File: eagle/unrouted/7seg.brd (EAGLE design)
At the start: 43.2 x 33 mm, 14 parts, among them J1 CONN-8P, J2 CONN-4P-4P

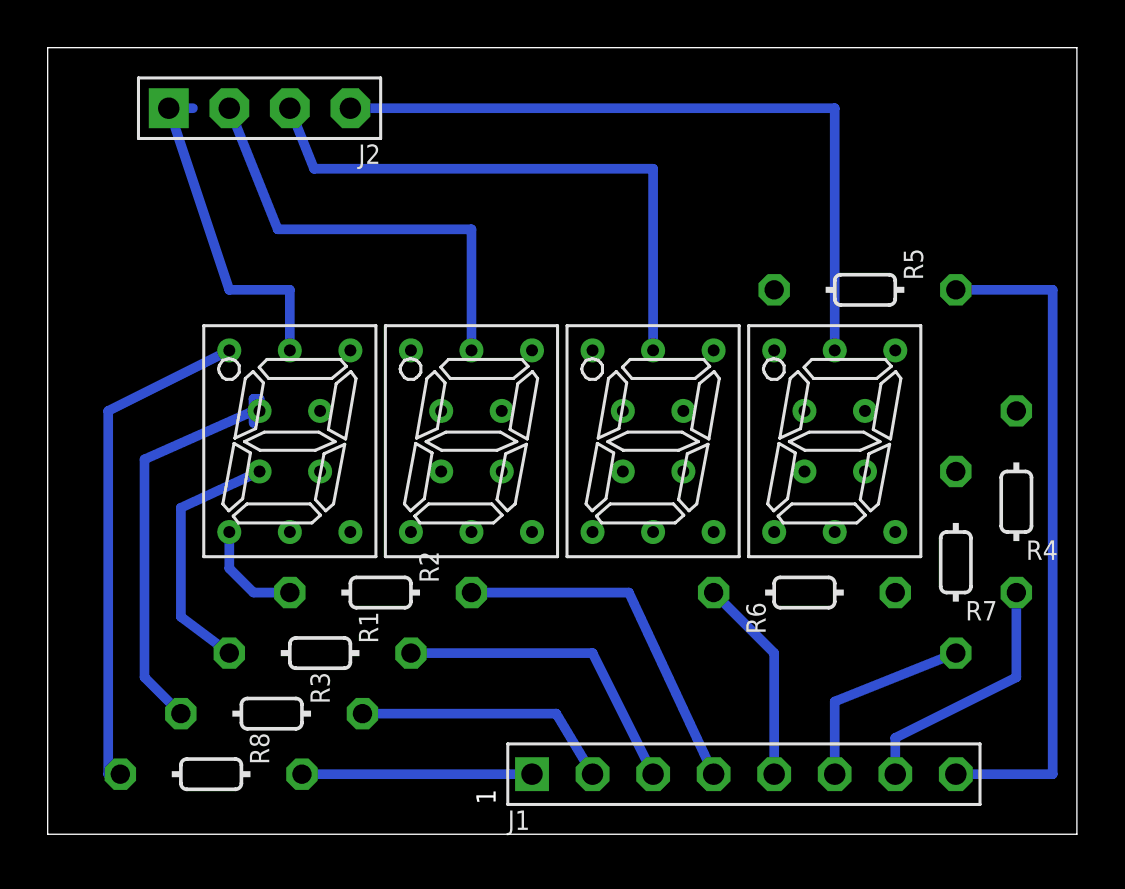
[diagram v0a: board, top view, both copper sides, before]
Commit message: ...
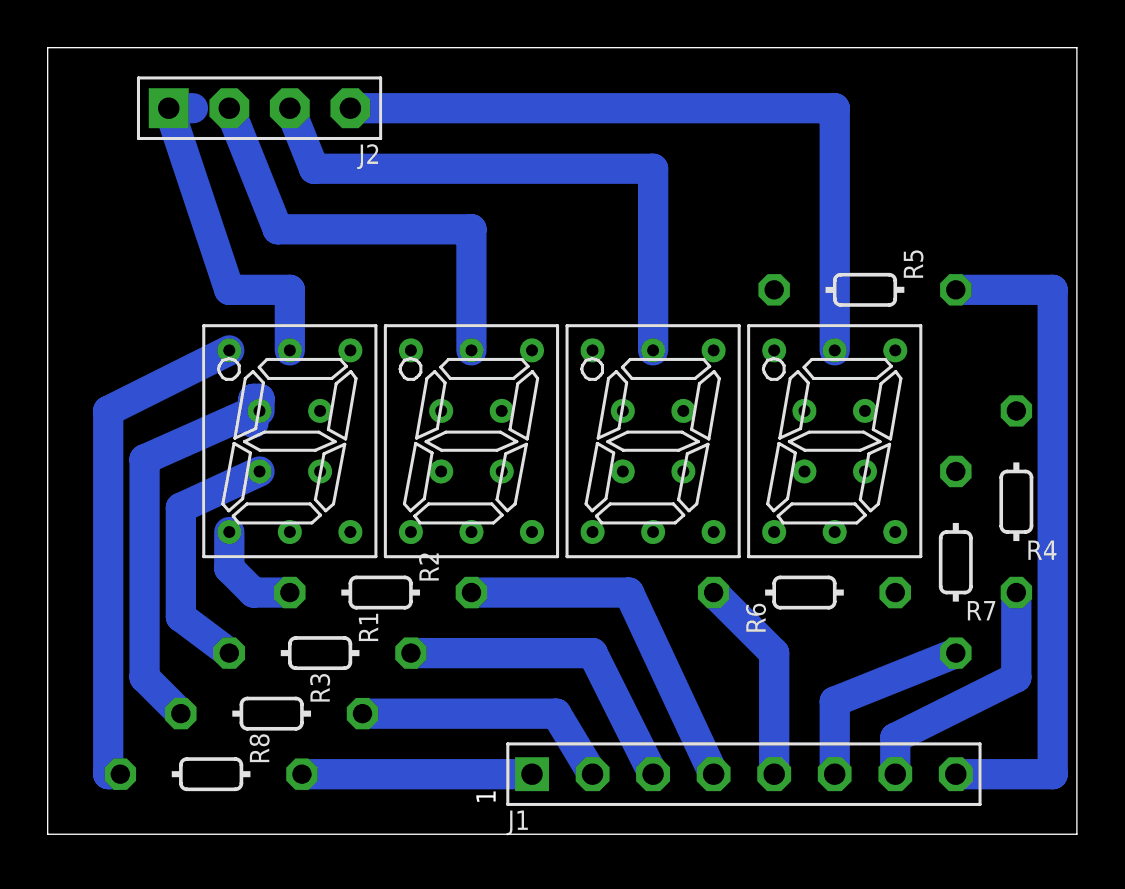
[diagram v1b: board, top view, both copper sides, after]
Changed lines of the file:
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@@
 <contactref element="U$1" pad="8"/>
 <contactref element="J2" pad="1"/>
-<wire x1="6.096" y1="30.48" x2="5.08" y2="30.48" width="0.4064" layer="16"/>
-<wire x1="5.08" y1="30.48" x2="7.62" y2="22.86" width="0.4064" layer="16"/>
-<wire x1="7.62" y1="22.86" x2="10.16" y2="22.86" width="0.4064" layer="16"/>
-<wire x1="10.16" y1="22.86" x2="10.16" y2="20.32" width="0.4064" layer="16"/>
+<wire x1="6.096" y1="30.48" x2="5.08" y2="30.48" width="1.27" layer="16"/>
+<wire x1="5.08" y1="30.48" x2="7.62" y2="22.86" width="1.27" layer="16"/>
+<wire x1="7.62" y1="22.86" x2="10.16" y2="22.86" width="1.27" layer="16"/>
+<wire x1="10.16" y1="22.86" x2="10.16" y2="20.32" width="1.27" layer="16"/>
 <wire x1="10.16" y1="12.7" x2="10.16" y2="20.32" width="0" layer="19" extent="1-1"/>
 </signal>
@@
 <contactref element="U$2" pad="8"/>
 <contactref element="J2" pad="2"/>
-<wire x1="7.62" y1="30.48" x2="9.652" y2="25.4" width="0.4064" layer="16"/>
-<wire x1="9.652" y1="25.4" x2="17.78" y2="25.4" width="0.4064" layer="16"/>
-<wire x1="17.78" y1="25.4" x2="17.78" y2="20.32" width="0.4064" layer="16"/>
+<wire x1="7.62" y1="30.48" x2="9.652" y2="25.4" width="1.27" layer="16"/>
+<wire x1="9.652" y1="25.4" x2="17.78" y2="25.4" width="1.27" layer="16"/>
+<wire x1="17.78" y1="25.4" x2="17.78" y2="20.32" width="1.27" layer="16"/>
 <wire x1="17.78" y1="12.7" x2="17.78" y2="20.32" width="0" layer="19" extent="1-1"/>
 </signal>
@@
 <contactref element="U$3" pad="8"/>
 <contactref element="J2" pad="3"/>
-<wire x1="10.16" y1="30.48" x2="11.176" y2="27.94" width="0.4064" layer="16"/>
-<wire x1="11.176" y1="27.94" x2="25.4" y2="27.94" width="0.4064" layer="16"/>
-<wire x1="25.4" y1="27.94" x2="25.4" y2="20.32" width="0.4064" layer="16"/>
+<wire x1="10.16" y1="30.48" x2="11.176" y2="27.94" width="1.27" layer="16"/>
+<wire x1="11.176" y1="27.94" x2="25.4" y2="27.94" width="1.27" layer="16"/>
+<wire x1="25.4" y1="27.94" x2="25.4" y2="20.32" width="1.27" layer="16"/>
 <wire x1="25.4" y1="20.32" x2="25.4" y2="12.7" width="0" layer="19" extent="1-1"/>
 </signal>
@@
 <contactref element="U$4" pad="8"/>
 <contactref element="J2" pad="4"/>
-<wire x1="12.7" y1="30.48" x2="33.02" y2="30.48" width="0.4064" layer="16"/>
-<wire x1="33.02" y1="30.48" x2="33.02" y2="20.32" width="0.4064" layer="16"/>
+<wire x1="12.7" y1="30.48" x2="33.02" y2="30.48" width="1.27" layer="16"/>
+<wire x1="33.02" y1="30.48" x2="33.02" y2="20.32" width="1.27" layer="16"/>
 <wire x1="33.02" y1="20.32" x2="33.02" y2="12.7" width="0" layer="19" extent="1-1"/>
 </signal>
@@
 <contactref element="U$1" pad="5"/>
 <contactref element="R8" pad="2"/>
-<wire x1="3.048" y1="2.54" x2="2.54" y2="2.54" width="0.4064" layer="16"/>
-<wire x1="2.54" y1="2.54" x2="2.54" y2="17.78" width="0.4064" layer="16"/>
-<wire x1="2.54" y1="17.78" x2="7.62" y2="20.32" width="0.4064" layer="16"/>
+<wire x1="3.048" y1="2.54" x2="2.54" y2="2.54" width="1.27" layer="16"/>
+<wire x1="2.54" y1="2.54" x2="2.54" y2="17.78" width="1.27" layer="16"/>
+<wire x1="2.54" y1="17.78" x2="7.62" y2="20.32" width="1.27" layer="16"/>
 <wire x1="22.86" y1="20.32" x2="30.48" y2="20.32" width="0" layer="19" extent="1-1"/>
 <wire x1="15.24" y1="20.32" x2="22.86" y2="20.32" width="0" layer="19" extent="1-1"/>
@@
 <contactref element="U$2" pad="7"/>
 <contactref element="R1" pad="2"/>
-<wire x1="8.89" y1="15.24" x2="5.588" y2="13.716" width="0.4064" layer="16"/>
-<wire x1="5.588" y1="13.716" x2="5.588" y2="9.144" width="0.4064" layer="16"/>
-<wire x1="5.588" y1="9.144" x2="7.62" y2="7.62" width="0.4064" layer="16"/>
+<wire x1="8.89" y1="15.24" x2="5.588" y2="13.716" width="1.27" layer="16"/>
+<wire x1="5.588" y1="13.716" x2="5.588" y2="9.144" width="1.27" layer="16"/>
+<wire x1="5.588" y1="9.144" x2="7.62" y2="7.62" width="1.27" layer="16"/>
 <wire x1="24.13" y1="15.24" x2="31.75" y2="15.24" width="0" layer="19" extent="1-1"/>
 <wire x1="16.51" y1="15.24" x2="24.13" y2="15.24" width="0" layer="19" extent="1-1"/>
@@
 <contactref element="U$2" pad="6"/>
 <contactref element="R2" pad="2"/>
-<wire x1="10.16" y1="10.16" x2="8.636" y2="10.16" width="0.4064" layer="16"/>
-<wire x1="8.636" y1="10.16" x2="7.62" y2="11.176" width="0.4064" layer="16"/>
-<wire x1="7.62" y1="11.176" x2="7.62" y2="12.7" width="0.4064" layer="16"/>
+<wire x1="10.16" y1="10.16" x2="8.636" y2="10.16" width="1.27" layer="16"/>
+<wire x1="8.636" y1="10.16" x2="7.62" y2="11.176" width="1.27" layer="16"/>
+<wire x1="7.62" y1="11.176" x2="7.62" y2="12.7" width="1.27" layer="16"/>
 <wire x1="22.86" y1="12.7" x2="30.48" y2="12.7" width="0" layer="19" extent="1-1"/>
 <wire x1="15.24" y1="12.7" x2="22.86" y2="12.7" width="0" layer="19" extent="1-1"/>
@@
 <contactref element="U$2" pad="4"/>
 <contactref element="R3" pad="2"/>
-<wire x1="5.588" y1="5.08" x2="4.064" y2="6.604" width="0.4064" layer="16"/>
-<wire x1="4.064" y1="6.604" x2="4.064" y2="15.748" width="0.4064" layer="16"/>
-<wire x1="4.064" y1="15.748" x2="8.636" y2="17.78" width="0.4064" layer="16"/>
-<wire x1="8.636" y1="17.78" x2="8.636" y2="17.272" width="0.4064" layer="16"/>
-<wire x1="8.636" y1="17.78" x2="8.636" y2="18.288" width="0.4064" layer="16"/>
-<wire x1="8.636" y1="18.288" x2="8.89" y2="18.288" width="0.4064" layer="16"/>
-<wire x1="8.89" y1="18.288" x2="8.89" y2="17.78" width="0.4064" layer="16"/>
+<wire x1="5.588" y1="5.08" x2="4.064" y2="6.604" width="1.27" layer="16"/>
+<wire x1="4.064" y1="6.604" x2="4.064" y2="15.748" width="1.27" layer="16"/>
+<wire x1="4.064" y1="15.748" x2="8.636" y2="17.78" width="1.27" layer="16"/>
+<wire x1="8.636" y1="17.78" x2="8.636" y2="17.272" width="1.27" layer="16"/>
+<wire x1="8.636" y1="17.78" x2="8.636" y2="18.288" width="1.27" layer="16"/>
+<wire x1="8.636" y1="18.288" x2="8.89" y2="18.288" width="1.27" layer="16"/>
+<wire x1="8.89" y1="18.288" x2="8.89" y2="17.78" width="1.27" layer="16"/>
 <wire x1="24.13" y1="17.78" x2="31.75" y2="17.78" width="0" layer="19" extent="1-1"/>
 <wire x1="16.51" y1="17.78" x2="24.13" y2="17.78" width="0" layer="19" extent="1-1"/>
@@
 <contactref element="R1" pad="1"/>
 <contactref element="J1" pad="3"/>
-<wire x1="15.24" y1="7.62" x2="22.86" y2="7.62" width="0.4064" layer="16"/>
-<wire x1="22.86" y1="7.62" x2="25.4" y2="2.54" width="0.4064" layer="16"/>
+<wire x1="15.24" y1="7.62" x2="22.86" y2="7.62" width="1.27" layer="16"/>
+<wire x1="22.86" y1="7.62" x2="25.4" y2="2.54" width="1.27" layer="16"/>
 </signal>
 <signal name="N$2">
 <contactref element="R2" pad="1"/>
 <contactref element="J1" pad="4"/>
-<wire x1="17.78" y1="10.16" x2="24.384" y2="10.16" width="0.4064" layer="16"/>
-<wire x1="24.384" y1="10.16" x2="27.94" y2="2.54" width="0.4064" layer="16"/>
+<wire x1="17.78" y1="10.16" x2="24.384" y2="10.16" width="1.27" layer="16"/>
+<wire x1="24.384" y1="10.16" x2="27.94" y2="2.54" width="1.27" layer="16"/>
 </signal>
 <signal name="N$3">
 <contactref element="R3" pad="1"/>
 <contactref element="J1" pad="2"/>
-<wire x1="13.208" y1="5.08" x2="21.336" y2="5.08" width="0.4064" layer="16"/>
-<wire x1="21.336" y1="5.08" x2="22.86" y2="2.54" width="0.4064" layer="16"/>
+<wire x1="13.208" y1="5.08" x2="21.336" y2="5.08" width="1.27" layer="16"/>
+<wire x1="21.336" y1="5.08" x2="22.86" y2="2.54" width="1.27" layer="16"/>
 </signal>
 <signal name="N$4">
 <contactref element="R4" pad="1"/>
 <contactref element="J1" pad="7"/>
-<wire x1="35.56" y1="2.54" x2="35.56" y2="4.064" width="0.4064" layer="16"/>
-<wire x1="35.56" y1="4.064" x2="40.64" y2="6.604" width="0.4064" layer="16"/>
-<wire x1="40.64" y1="6.604" x2="40.64" y2="10.16" width="0.4064" layer="16"/>
+<wire x1="35.56" y1="2.54" x2="35.56" y2="4.064" width="1.27" layer="16"/>
+<wire x1="35.56" y1="4.064" x2="40.64" y2="6.604" width="1.27" layer="16"/>
+<wire x1="40.64" y1="6.604" x2="40.64" y2="10.16" width="1.27" layer="16"/>
 </signal>
 <signal name="N$5">
 <contactref element="R5" pad="1"/>
 <contactref element="J1" pad="8"/>
-<wire x1="38.1" y1="2.54" x2="42.164" y2="2.54" width="0.4064" layer="16"/>
-<wire x1="42.164" y1="2.54" x2="42.164" y2="22.86" width="0.4064" layer="16"/>
-<wire x1="42.164" y1="22.86" x2="38.1" y2="22.86" width="0.4064" layer="16"/>
+<wire x1="38.1" y1="2.54" x2="42.164" y2="2.54" width="1.27" layer="16"/>
+<wire x1="42.164" y1="2.54" x2="42.164" y2="22.86" width="1.27" layer="16"/>
+<wire x1="42.164" y1="22.86" x2="38.1" y2="22.86" width="1.27" layer="16"/>
 </signal>
 <signal name="N$6">
 <contactref element="R6" pad="1"/>
 <contactref element="J1" pad="5"/>
-<wire x1="27.94" y1="10.16" x2="30.48" y2="7.62" width="0.4064" layer="16"/>
-<wire x1="30.48" y1="7.62" x2="30.48" y2="2.54" width="0.4064" layer="16"/>
+<wire x1="27.94" y1="10.16" x2="30.48" y2="7.62" width="1.27" layer="16"/>
+<wire x1="30.48" y1="7.62" x2="30.48" y2="2.54" width="1.27" layer="16"/>
 </signal>
 <signal name="N$7">
 <contactref element="R7" pad="1"/>
 <contactref element="J1" pad="6"/>
-<wire x1="33.02" y1="2.54" x2="33.02" y2="5.588" width="0.4064" layer="16"/>
-<wire x1="33.02" y1="5.588" x2="38.1" y2="7.62" width="0.4064" layer="16"/>
+<wire x1="33.02" y1="2.54" x2="33.02" y2="5.588" width="1.27" layer="16"/>
+<wire x1="33.02" y1="5.588" x2="38.1" y2="7.62" width="1.27" layer="16"/>
 </signal>
 <signal name="N$8">
 <contactref element="R8" pad="1"/>
 <contactref element="J1" pad="1"/>
-<wire x1="10.668" y1="2.54" x2="20.32" y2="2.54" width="0.4064" layer="16"/>
+<wire x1="10.668" y1="2.54" x2="20.32" y2="2.54" width="1.27" layer="16"/>
 </signal>
 </signals>
